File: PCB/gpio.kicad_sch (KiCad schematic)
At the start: 0 parts

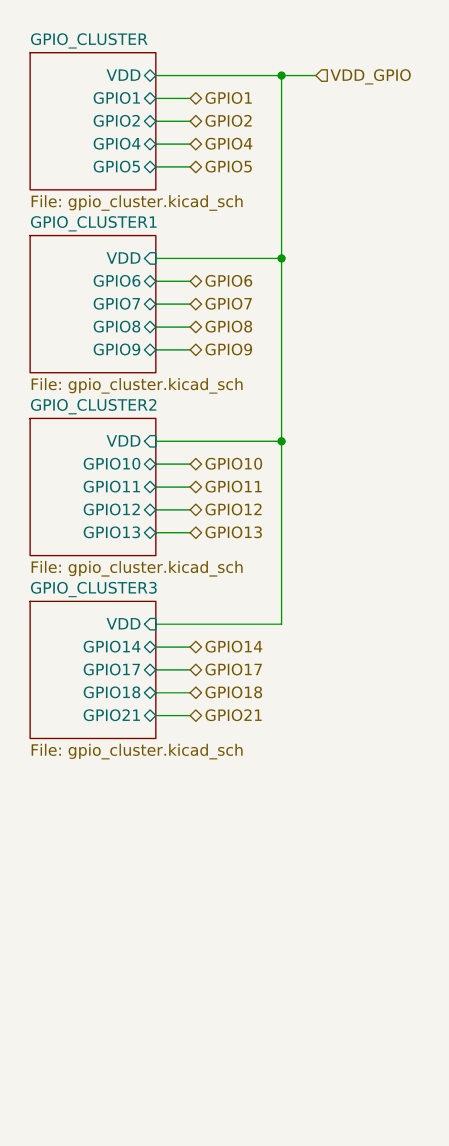
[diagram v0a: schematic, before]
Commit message: yeah just read the journal son
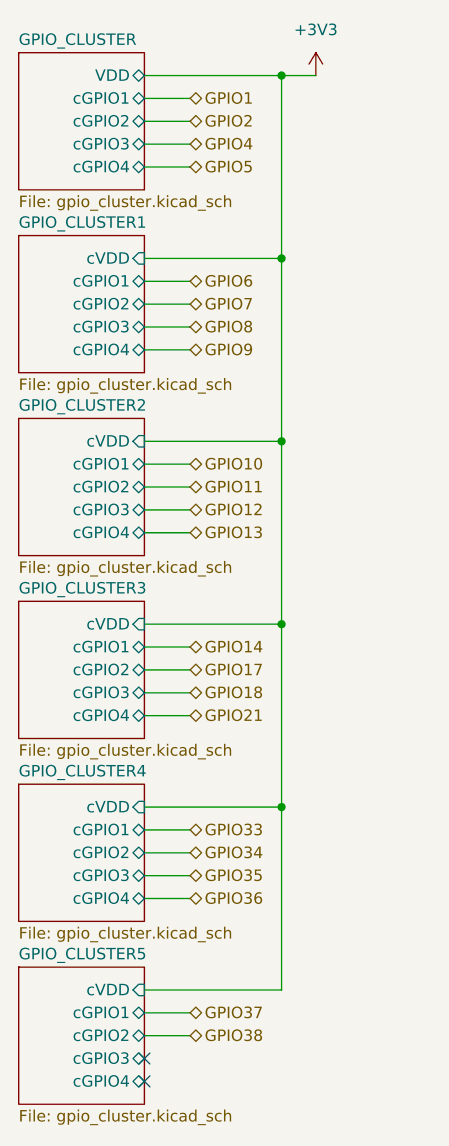
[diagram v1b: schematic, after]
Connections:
- no-connect marks 0 -> 2
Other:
- added sheet GPIO_CLUSTER4 (gpio_cluster.kicad_sch)
- added sheet GPIO_CLUSTER5 (gpio_cluster.kicad_sch)
- sheet GPIO_CLUSTER ports: added cGPIO1, cGPIO2, cGPIO3, cGPIO4; removed GPIO1, GPIO2, GPIO4, GPIO5
- sheet GPIO_CLUSTER1 ports: added cGPIO1, cGPIO2, cGPIO3, cGPIO4, cVDD; removed GPIO6, GPIO7, GPIO8, GPIO9, VDD
- sheet GPIO_CLUSTER2 ports: added cGPIO1, cGPIO2, cGPIO3, cGPIO4, cVDD; removed GPIO10, GPIO11, GPIO12, GPIO13, VDD
- sheet GPIO_CLUSTER3 ports: added cGPIO1, cGPIO2, cGPIO3, cGPIO4, cVDD; removed GPIO14, GPIO17, GPIO18, GPIO21, VDD
